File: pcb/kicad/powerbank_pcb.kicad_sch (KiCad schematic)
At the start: 30 parts, among them J1 USB_C_OUT, J2 USB_C_IN, U1 TPS61022, U2 IP2312-ESOP8

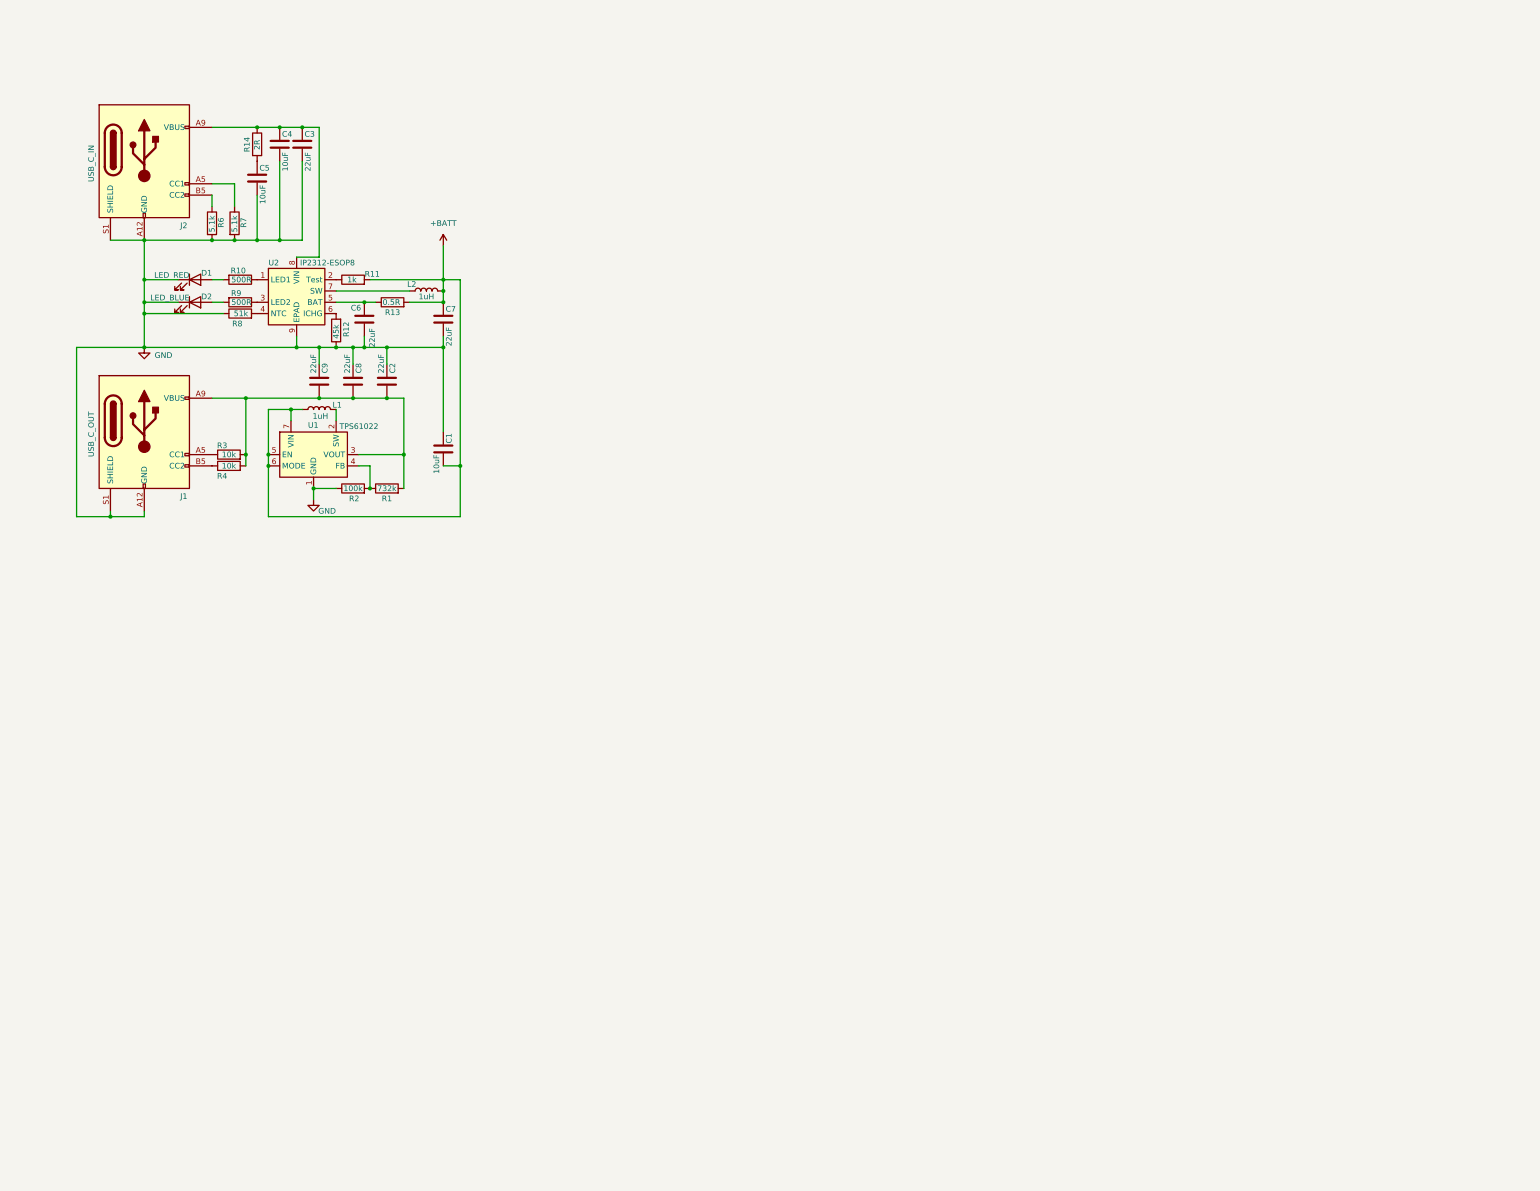
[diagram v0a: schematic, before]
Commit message: first draft
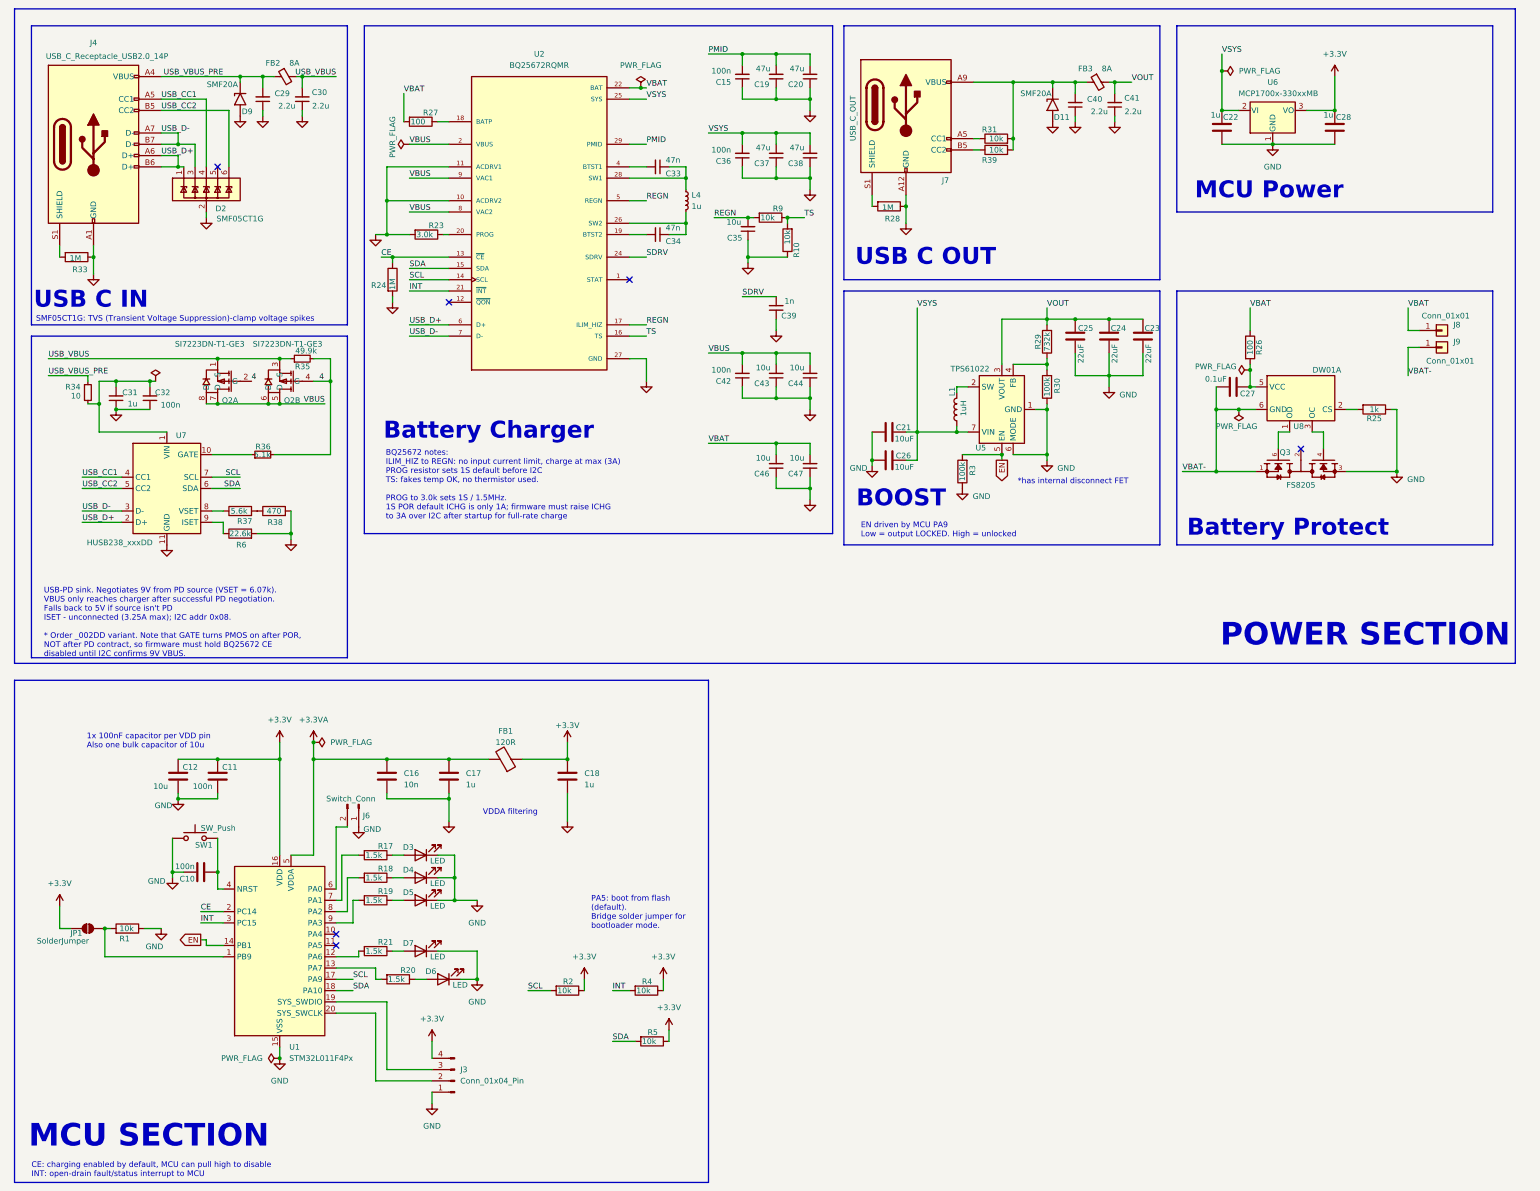
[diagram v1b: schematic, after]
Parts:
- removed C1, C4, C5: 10uF, Capacitor_SMD:C_0805_2012Metric_Pad1.18x1.45mm_HandSolder, symbol Device:C
- removed C2: 22uF, symbol Device:C
- removed C3, C6, C7, C8, C9: 22uF, Capacitor_SMD:C_0805_2012Metric_Pad1.18x1.45mm_HandSolder, symbol Device:C
- removed D1: LED_RED, LED_SMD:LED_0805_2012Metric_Pad1.15x1.40mm_HandSolder, symbol Device:LED
- removed D2: LED_BLUE, LED_SMD:LED_0805_2012Metric_Pad1.15x1.40mm_HandSolder, symbol Device:LED
- removed J1: USB_C_OUT, Connector_USB:USB_C_Receptacle_GCT_USB4125-xx-x_6P_TopMnt_Horizontal, symbol Connector:USB_C_Receptacle_PowerOnly_6P
- removed J2: USB_C_IN, Connector_USB:USB_C_Receptacle_GCT_USB4125-xx-x_6P_TopMnt_Horizontal, symbol Connector:USB_C_Receptacle_PowerOnly_6P
- removed L2: 1uH, Inductor_SMD:L_Coilcraft_XxL4030, symbol Device:L
- removed R11: 1k, Resistor_SMD:R_0805_2012Metric_Pad1.20x1.40mm_HandSolder, symbol Device:R
- removed R12: 45k, Resistor_SMD:R_0805_2012Metric_Pad1.20x1.40mm_HandSolder, symbol Device:R
- removed R13: 0.5R, Resistor_SMD:R_0805_2012Metric_Pad1.20x1.40mm_HandSolder, symbol Device:R
- removed R14: 2R, Resistor_SMD:R_0805_2012Metric_Pad1.20x1.40mm_HandSolder, symbol Device:R
- removed R7: 5.1k, Resistor_SMD:R_0805_2012Metric_Pad1.20x1.40mm_HandSolder, symbol Device:R
- removed R8: 51k, Resistor_SMD:R_0805_2012Metric_Pad1.20x1.40mm_HandSolder, symbol Device:R
- removed U1: TPS61022, Package_DFN_QFN:Texas_RWU0007A_VQFN-7_2x2mm_P0.5mm, symbol Converter_DCDC:TPS61022
- removed U2: IP2312-ESOP8, Package_SO:SOIC-8-1EP_3.9x4.9mm_P1.27mm_EP2.41x3.3mm_ThermalVias, symbol Battery_Management:IP2312-ESOP8
- added C10, C11: 100n, Capacitor_SMD:C_0603_1608Metric, symbol Device:C
- added C12: 10u, Capacitor_SMD:C_0805_2012Metric, symbol Device:C
- added C15, C36: 100n, Capacitor_SMD:C_0805_2012Metric, symbol Device:C_Small
- added C16: 10n, Capacitor_SMD:C_0603_1608Metric, symbol Device:C
- added C17, C18, C22, C28: 1u, Capacitor_SMD:C_0603_1608Metric, symbol Device:C
- added C19, C20, C37, C38: 47u, Capacitor_SMD:C_0805_2012Metric, symbol Device:C_Small
- added C21, C26: 10uF, Capacitor_SMD:C_0805_2012Metric, symbol Device:C
- added C23, C24, C25: 22uF, Capacitor_SMD:C_0805_2012Metric, symbol Device:C
- added C27: 0.1uF, Capacitor_SMD:C_0603_1608Metric, symbol Device:C
- added C29, C30, C40, C41: 2.2u, Capacitor_SMD:C_0603_1608Metric, symbol Device:C_Small
- added C31: 1u, Capacitor_SMD:C_0603_1608Metric, symbol Device:C_Small
- added C32, C42: 100n, Capacitor_SMD:C_0603_1608Metric, symbol Device:C_Small
- added C33, C34: 47n, Capacitor_SMD:C_0603_1608Metric, symbol Device:C_Small
- added C35, C43, C44, C46, C47: 10u, Capacitor_SMD:C_0805_2012Metric, symbol Device:C_Small
- added C39: 1n, Capacitor_SMD:C_0402_1005Metric, symbol Device:C_Small
- added D11, D9: SMF20A, Diode_SMD:D_SMF, symbol Diode:SMF20A
- added D2: SMF05CT1G, Package_TO_SOT_SMD:SOT-23-6, symbol Power_Protection:ESDA6V1-5SC6
- added D3, D4, D5, D6, D7: LED, LED_SMD:LED_0805_2012Metric, symbol Device:LED
- added FB1: 120R, Inductor_SMD:L_0805_2012Metric, symbol Device:FerriteBead
- added FB2, FB3: 8A, Inductor_SMD:L_0805_2012Metric, symbol Device:FerriteBead_Small
- added J3: Conn_01x04_Pin, Connector_PinHeader_2.54mm:PinHeader_1x04_P2.54mm_Vertical, symbol Connector:Conn_01x04_Pin
- added J4: USB_C_Receptacle_USB2.0_14P, Connector_USB:USB_C_Receptacle_GCT_USB4105-xx-A_16P_TopMnt_Horizontal, symbol Connector:USB_C_Receptacle_USB2.0_14P
- added J6: Switch_Conn, Connector_PinHeader_2.54mm:PinHeader_1x02_P2.54mm_Vertical, symbol Connector:Conn_01x02_Pin
- added J7: USB_C_OUT, Connector_USB:USB_C_Receptacle_GCT_USB4125-xx-x_6P_TopMnt_Horizontal, symbol Connector:USB_C_Receptacle_PowerOnly_6P
- added J8, J9: Conn_01x01, TestPoint:TestPoint_THTPad_2.0x2.0mm_Drill1.0mm, symbol Connector_Generic:Conn_01x01
- added JP1: SolderJumper, Jumper:SolderJumper-2_P1.3mm_Open_RoundedPad1.0x1.5mm, symbol Jumper:SolderJumper_2_Open
- added L4: 1u, Inductor_SMD:L_Changjiang_FXL0530, symbol Device:L_Small
- added Q2: SI7223DN-T1-GE3, si7223dn:PDFN3333-8_L3.1-W3.1-P0.65-LS3.4-BL-EP, symbol si7223dn:SI7223DN-T1-GE3
- added Q3: FS8205, FS8205:SOT95P280X145-6N, symbol FS8205:FS8205
- added R17, R18, R19, R20, R21: 1.5k, Resistor_SMD:R_0603_1608Metric, symbol Device:R
- added R23: 3.0k, Resistor_SMD:R_0603_1608Metric, symbol Device:R
- added R24, R28, R33: 1M, Resistor_SMD:R_0603_1608Metric, symbol Device:R
- added R25: 1k, Resistor_SMD:R_0603_1608Metric, symbol Device:R
- added R26, R27: 100, Resistor_SMD:R_0603_1608Metric, symbol Device:R
- added R29: 732k, Resistor_SMD:R_0603_1608Metric, symbol Device:R
- added R30: 100k, Resistor_SMD:R_0603_1608Metric, symbol Device:R
- added R31, R39, R5: 10k, Resistor_SMD:R_0603_1608Metric, symbol Device:R
- added R34: 10, Resistor_SMD:R_0603_1608Metric, symbol Device:R_Small
- added R35: 49.9k, Resistor_SMD:R_0603_1608Metric, symbol Device:R_Small
- added R36: 5.1k, Resistor_SMD:R_0603_1608Metric, symbol Device:R_Small
- added R37: 5.6k, Resistor_SMD:R_0603_1608Metric, symbol Device:R
- added R38: 470, Resistor_SMD:R_0603_1608Metric, symbol Device:R
- added SW1: SW_Push, Button_Switch_SMD:SW_SPST_B3U-1000P, symbol Switch:SW_Push
- added U1: STM32L011F4Px, Package_SO:TSSOP-20_4.4x6.5mm_P0.65mm, symbol MCU_ST_STM32L0:STM32L011F4Px
- added U2: BQ25672RQMR, BQ25672RQMR:IC_BQ25672RQMR, symbol BQ25672RQMR:BQ25672RQMR
- added U5: TPS61022, Package_DFN_QFN:Texas_RWU0007A_VQFN-7_2x2mm_P0.5mm, symbol Converter_DCDC:TPS61022
- added U6: MCP1700x-330xxMB, Package_TO_SOT_SMD:SOT-89-3, symbol Regulator_Linear:MCP1700x-330xxMB
- added U7: HUSB238_xxxDD, Package_DFN_QFN:WDFN-10-1EP_3x3mm_P0.5mm_EP1.8x2.5mm, symbol Interface_USB:HUSB238_xxxDD
- added U8: DW01A, Package_TO_SOT_SMD:SOT-23-6, symbol Battery_Management:DW01A
- L1: footprint Inductor_SMD:L_Coilcraft_XxL4030 -> Inductor_SMD:L_Coilcraft_XAL7030-102
- R1: value 732k -> 10k; footprint Resistor_SMD:R_0805_2012Metric_Pad1.20x1.40mm_HandSolder -> Resistor_SMD:R_0603_1608Metric
- R10, R9: value 500R -> 10k; footprint Resistor_SMD:R_0805_2012Metric_Pad1.20x1.40mm_HandSolder -> Resistor_SMD:R_0805_2012Metric
- R2: value 100k -> 10k; footprint Resistor_SMD:R_0805_2012Metric_Pad1.20x1.40mm_HandSolder -> Resistor_SMD:R_0603_1608Metric
- R3: value 10k -> 100k; footprint Resistor_SMD:R_0805_2012Metric_Pad1.20x1.40mm_HandSolder -> Resistor_SMD:R_0603_1608Metric
- R4: footprint Resistor_SMD:R_0805_2012Metric_Pad1.20x1.40mm_HandSolder -> Resistor_SMD:R_0603_1608Metric
- R6: value 5.1k -> 22.6k; footprint Resistor_SMD:R_0805_2012Metric_Pad1.20x1.40mm_HandSolder -> Resistor_SMD:R_0603_1608Metric
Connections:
- net GND: now also R1.1, R10.1, R3.1, C10.1, C11.2, C12.2, C15.1, C16.2, C17.2, C18.2, C19.1, C20.1, C21.2, C22.2, C23.1, C24.1, C25.1, C26.2, C28.2, C29.1, C30.1, C31.1, C32.1, C35.1, C36.1, C37.1, C38.1, C39.1, C40.1, C41.1, C42.1, C43.1, C44.1, C46.1, C47.1, D11.2 (A2), D2.2 (GND), D3.1 (K), D4.1 (K), D5.1 (K), D6.1 (K), D7.1 (K), D9.2 (A2), J3.1 (Pin_1), J4.A1 (GND), J4.A12 (GND), J4.B1 (GND), J4.B12 (GND), J6.1 (Pin_1), J7.A12 (GND), J7.B12 (GND), Q3.3, R23.2, R24.2, R25.1, R28.1, R30.1, R33.1, R38.2, SW1.1, U1.15 (VSS), U2.10 (ACDRV2), U2.11 (ACDRV1), U2.27 (GND), U5.1 (GND), U5.6 (MODE), U6.1 (GND), U7.11 (GND); no longer R2.1
- net SCL: now reaches R2.2
- net SCL: now also U1.17 (PA9), U2.14 (SCL), U7.7 (SCL); no longer R1.1
- net at R6.1: now also U7.9 (ISET)
- net +3.3V: now reaches R4.1
- net +3.3V: now also R2.1, C11.1, C12.1, C18.1, C28.1, FB1.1, J3.4 (Pin_4), JP1.1 (A), R5.1, U1.16 (VDD), U6.3 (VO)
- net at L1.2: now also U5.2 (SW)
- net TS: now reaches R10.2
- net TS: now also R9.1, U2.16 (TS)
- net REGN: now reaches R9.2
- net REGN: now also C35.2, U2.17 (ILIM_HIZ), U2.5 (REGN)
- net +BATT renamed VSYS
- net VSYS: now also C21.1, C22.1, C26.1, C36.2, C37.2, C38.2, U2.25 (SYS), U5.7 (VIN), U6.2 (VI)
- new net: J4.S1 (SHIELD), R33.2
- new net: R36.1, U7.10 (GATE)
- new net: C31.2, C32.2, R34.2, U7.1 (VIN)
- new net: J3.2 (Pin_2), U1.20 (PA14)
- new net: J3.3 (Pin_3), U1.19 (PA13)
- new net: R23.1, U2.20 (PROG)
- new net: D3.2 (A), R17.1
- new net: R17.2, U1.7 (PA1)
- new net: R37.1, U7.8 (VSET)
- new net: R37.2, R38.1
- new net: C40.2, D11.1 (A1), FB3.1, J7.A9 (VBUS), J7.B9 (VBUS), R31.2, R39.2
- new net: R27.1, U2.18 (BATP)
- new net: C34.2, U2.19 (BTST2)
- new net: C34.1, L4.2, U2.26 (SW2)
- new net: C33.1, L4.1, U2.28 (SW1)
- new net: C33.2, U2.4 (BTST1)
- new net: C27.1, R26.2, U8.5 (VCC)
- new net: D5.2 (A), R19.1
- new net: Q3.2, Q3.5
- new net: Q3.4, U8.3 (OC)
- new net: Q3.6, U8.1 (OD)
- new net: R25.2, U8.2 (CS)
- new net: R29.1, R30.2, U5.4 (FB)
- new net: J7.A5 (CC1), R31.1
- new net: JP1.2 (B), R1.2, U1.1 (PB9)
- new net: R21.2, U1.12 (PA6)
- new net: R20.2, U1.13 (PA7)
- new net: C10.2, SW1.2, U1.4 (NRST)
- new net: J6.2 (Pin_2), U1.6 (PA0)
- new net: R18.2, U1.8 (PA2)
- new net: R19.2, U1.9 (PA3)
- new net: D4.2 (A), R18.1
- new net: J7.B5 (CC2), R39.1
- new net: J7.S1 (SHIELD), R28.2
- new net: D7.2 (A), R21.1
- new net: D6.2 (A), R20.1
- new net +3.3VA: C16.1, C17.1, FB1.2, U1.5 (VDDA)
- new net 4: Q2.2 (G), Q2.4 (G), R35.2, R36.2
- new net BAT: C46.2, C47.2, J8.1 (Pin_1), R26.1, R27.2, U2.22 (BAT), U2.23 (BAT)
- new net CE: R24.1, U1.2 (PC14), U2.13 (~{CE})
- new net EN: R3.2, U1.14 (PB1), U5.5 (EN)
- new net INT: R4.2, U1.3 (PC15), U2.21 (~{INT})
- new net PMID: C15.2, C19.2, C20.2, U2.29 (PMID)
- new net SDA: R5.2, U1.18 (PA10), U2.15 (SDA), U7.6 (SDA)
- new net SDRV: C39.2, U2.24 (SDRV)
- new net USB_CC1: D2.4 (IO3), J4.A5 (CC1), U7.4 (CC1)
- new net USB_CC2: D2.6 (IO5), J4.B5 (CC2), U7.5 (CC2)
- new net USB_D+: D2.1 (IO1), J4.A6 (D+), J4.B6 (D+), U2.6 (D+), U7.2 (D+)
- new net USB_D-: D2.3 (IO2), J4.A7 (D-), J4.B7 (D-), U2.7 (D-), U7.3 (D-)
- new net USB_VBUS: C30.2, FB2.2, Q2.1 (S), Q2.3 (S), R35.1
- new net USB_VBUS_PRE: C29.2, D9.1 (A1), FB2.1, J4.A4 (VBUS), J4.A9 (VBUS), J4.B4 (VBUS), J4.B9 (VBUS), R34.1
- new net VBAT-: C27.2, J9.1 (Pin_1), Q3.1, U8.6 (GND)
- new net VBUS: C42.2, C43.2, C44.2, Q2.5 (D), Q2.6 (D), Q2.7 (D), Q2.8 (D), U2.2 (VBUS), U2.3 (VBUS), U2.8 (VAC2), U2.9 (VAC1)
- new net VOUT: C23.2, C24.2, C25.2, C41.2, FB3.2, R29.2, U5.3 (VOUT)
- no-connect marks 0 -> 6
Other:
- note added: "*has internal disconnect FET"
- note added: "1x 100nF capacitor per VDD pin Also one bulk capacitor of 10u"
- note added: "BOOST"
- note added: "BQ25672 notes: ILIM_HIZ to REGN: no input current limit, charge at max (3A) PROG resistor sets 1S default before I2C TS: fakes temp OK, no thermistor used. PROG to 3.0k sets 1S / 1.5MHz. 1S POR default ICHG is only 1A; firmware must raise ICHG to 3A over I2C after startup for full-rate charge"
- note added: "Battery Charger"
- note added: "Battery Protect"
- note added: "CE: charging enabled by default, MCU can pull high to disable INT: open-drain fault/status interrupt to MCU"
- note added: "EN driven by MCU PA9 Low = output LOCKED. High = unlocked"
- note added: "MCU Power"
- note added: "MCU SECTION"
- note added: "PA5: boot from flash (default). Bridge solder jumper for bootloader mode."
- note added: "POWER SECTION"
- note added: "SMF05CT1G: TVS (Transient Voltage Suppression)-clamp voltage spikes"
- note added: "USB C IN"
- note added: "USB C OUT"
- note added: "USB-PD sink. Negotiates 9V from PD source (VSET = 6.07k). VBUS only reaches charger after successful PD negotiation. Falls back to 5V if source isn't PD ISET - unconnected (3.25A max); I2C addr 0x08. * Order _002DD variant. Note that GATE turns PMOS on after POR, NOT after PD contract, so firmware must hold BQ25672 CE disabled until I2C confirms 9V VBUS."
- note added: "VDDA filtering"
- company: FL@NK -> (none)
- title: 3A/15W Powerbank PCB -> Powerbank PCB
